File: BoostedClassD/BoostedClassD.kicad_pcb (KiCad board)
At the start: 4 copper layers, 82.2 x 58.4 mm, 83 parts, among them IC1 BQ25185, IC2 ESP32-WROOM-32UE-N8R2, IC5 INA236, J1 SYSTEM CONNECTOR 1, J2 SYSTEM CONNECTOR 2, J3 SPK OUT, J4 PROG, J5 CC, Q1 DMG3415U, U1 TPS631000, U2 TAS2320, U3 TAS2120, U4 TPS7A2018, U5 ATtiny412

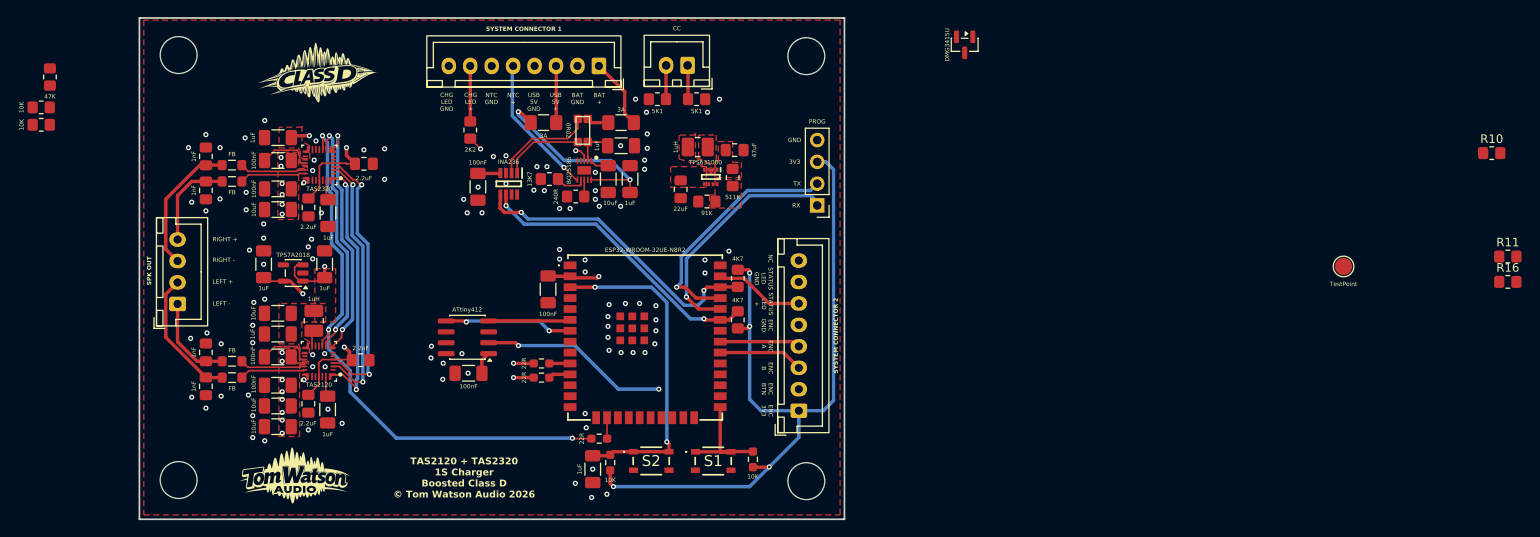
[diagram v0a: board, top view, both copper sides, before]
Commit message: more
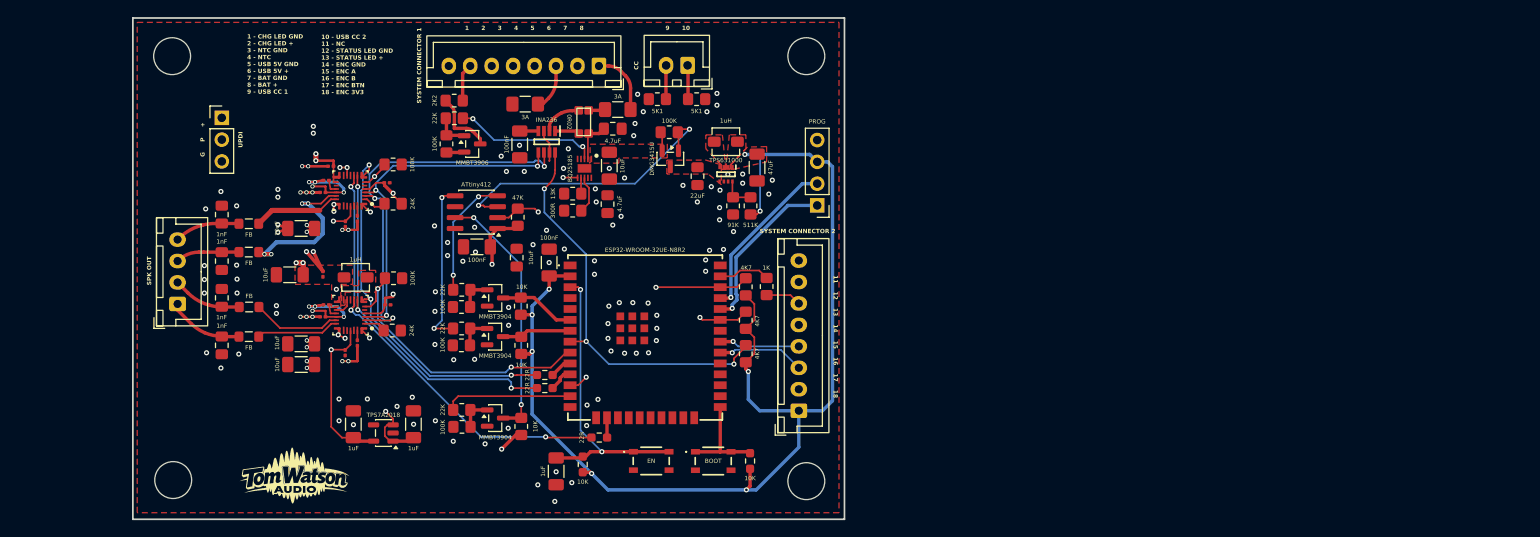
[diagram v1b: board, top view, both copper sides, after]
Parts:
- removed the G*** at (137.0, 78.2)
- removed R10: 0R*2, Resistor_SMD:R_0805_2012Metric_Pad1.20x1.40mm_HandSolder
- removed R11: 0R*3, Resistor_SMD:R_0805_2012Metric_Pad1.20x1.40mm_HandSolder
- removed TP1: TestPoint, TestPoint:TestPoint_Pad_D2.0mm
- added C32: 10uF, Capacitor_SMD:C_0805_2012Metric_Pad1.18x1.45mm_HandSolder, F.Cu at (160.3, 99.3)
- added J6: UPDI, Connector_PinHeader_2.54mm:PinHeader_1x03_P2.54mm_Vertical, F.Cu at (125.9, 83.0)
- added Q2: MMBT3904, Package_TO_SOT_SMD:SOT-23, F.Cu at (157.8, 104.0)
- added Q3: MMBT3904, Package_TO_SOT_SMD:SOT-23, F.Cu at (157.8, 108.5)
- added Q4: MMBT3904, Package_TO_SOT_SMD:SOT-23, F.Cu at (157.8, 118.0)
- added Q5: MMBT3906, Package_TO_SOT_SMD:SOT-23, F.Cu at (155.1, 86.0)
- added R22: 100K, Resistor_SMD:R_0805_2012Metric_Pad1.20x1.40mm_HandSolder, F.Cu at (145.9, 101.7)
- added R23: 100K, Resistor_SMD:R_0805_2012Metric_Pad1.20x1.40mm_HandSolder, F.Cu at (145.9, 88.4)
- added R24: 24K, Resistor_SMD:R_0805_2012Metric_Pad1.20x1.40mm_HandSolder, F.Cu at (145.8, 107.8)
- added R25: 24K, Resistor_SMD:R_0805_2012Metric_Pad1.20x1.40mm_HandSolder, F.Cu at (145.9, 93.0)
- added R26: 22K, Resistor_SMD:R_0805_2012Metric_Pad1.20x1.40mm_HandSolder, F.Cu at (153.9, 103.0)
- added R27: 100K, Resistor_SMD:R_0805_2012Metric_Pad1.20x1.40mm_HandSolder, F.Cu at (153.9, 105.1)
- added R28: 22K, Resistor_SMD:R_0805_2012Metric_Pad1.20x1.40mm_HandSolder, F.Cu at (153.9, 107.6)
- added R29: 100K, Resistor_SMD:R_0805_2012Metric_Pad1.20x1.40mm_HandSolder, F.Cu at (153.9, 109.5)
- added R30: 22K, Resistor_SMD:R_0805_2012Metric_Pad1.20x1.40mm_HandSolder, F.Cu at (153.9, 117.0)
- added R31: 100K, Resistor_SMD:R_0805_2012Metric_Pad1.20x1.40mm_HandSolder, F.Cu at (153.9, 119.0)
- added R32: 10K, Resistor_SMD:R_0805_2012Metric_Pad1.20x1.40mm_HandSolder, F.Cu at (160.8, 119.0)
- added R33: 4K7, Resistor_SMD:R_0805_2012Metric_Pad1.20x1.40mm_HandSolder, F.Cu at (187.0, 110.5)
- added R34: 1K, Resistor_SMD:R_0805_2012Metric_Pad1.20x1.40mm_HandSolder, F.Cu at (189.4, 102.7)
- added R35: 22K, Resistor_SMD:R_0805_2012Metric_Pad1.20x1.40mm_HandSolder, F.Cu at (153.0, 83.1)
- added R36: 100K, Resistor_SMD:R_0805_2012Metric_Pad1.20x1.40mm_HandSolder, F.Cu at (152.1, 86.0)
- C13, C14, C15, C16, C17, C18, C19, C20: footprint Capacitor_SMD:C_1206_3216Metric_Pad1.33x1.80mm_HandSolder -> Capacitor_SMD:C_0201_0603Metric
- C2: footprint Capacitor_SMD:C_0805_2012Metric_Pad1.18x1.45mm_HandSolder -> Capacitor_SMD:C_1206_3216Metric_Pad1.33x1.80mm_HandSolder
- C21, C22, C23, C24: footprint Capacitor_SMD:C_0805_2012Metric_Pad1.18x1.45mm_HandSolder -> Capacitor_SMD:C_0201_0603Metric
- C26, C27: value 1uF -> 4.7uF; footprint Capacitor_SMD:C_1206_3216Metric_Pad1.33x1.80mm_HandSolder -> Capacitor_SMD:C_0805_2012Metric_Pad1.18x1.45mm_HandSolder
- L1, L2: footprint Inductor_SMD:L_1008_2520Metric_Pad1.43x2.20mm_HandSolder -> Inductor_SMD:L_Vishay_IHLP-1212
- R17: value 240R -> 300R
- R18: value 13K7 -> 13K
- moved R16 99.3 mm to (178.1, 84.7), turned to 180 degrees
- moved R15 61.6 mm to (160.8, 109.5), turned to 90 degrees
- moved R14 60.5 mm to (160.8, 105.0), turned to 90 degrees
- moved R13 56.9 mm to (160.4, 94.6), turned to 90 degrees
- moved Q1 36.8 mm to (178.2, 87.8)
- moved U4 21.4 mm to (144.8, 119.7)
- moved C5 21.4 mm to (141.3, 118.7)
- moved C6 21.3 mm to (148.3, 118.7)
- moved C8 14.8 mm to (155.7, 98.0)
- moved U5 14.6 mm to (155.6, 94.0)
- moved C29 12.3 mm to (125.9, 99.7), turned to 90 degrees
- moved FB2 10.3 mm to (129.1, 98.7)
- moved C14 9.54 mm to (137.7, 106.2)
- moved C20 8.74 mm to (137.7, 101.2), turned to 90 degrees
- moved C16 8.50 mm to (141.7, 109.2)
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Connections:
- C2 pad 1: /ENC 3V3 -> /ESP3V3
- C22 pad 1: /Amplifiers/VDD1V8 -> /ESP3V3
- C24 pad 1: /Amplifiers/VDD1V8 -> /ESP3V3
- C25 pad 1: /CHGPOWER/BQ-SYS -> /BQ-SYS
- C3 pad 1: /ENC 3V3 -> /ESP3V3
- C7 pad 1: /ENC 3V3 -> /ESP3V3
- C8 pad 1: /Amplifiers/SYS -> /BQ-SYS
- IC1 pad 1: /CHGPOWER/BQ-SYS -> /BQ-SYS
- IC1 pad 3: Net-(IC1-STAT2) -> /CHGPOWER/STAT2_N
- IC2 pad 12: /Amplifiers/SDOUT -> /Amplifiers/AMP2320_SDZ
- IC2 pad 13: unconnected-(IC2-IO14-Pad13) -> /ESP32-ATTINY/SHUTDOWN_ACK
- IC2 pad 2: /ENC 3V3 -> /ESP3V3
- IC2 pad 37: /STATUS LED + -> Net-(IC2-IO23)
- IC2 pad 8: /ESP32-ATTINY/ALERT -> /ALERT_N
- IC2 pad 9: unconnected-(IC2-IO33-Pad9) -> /AMP2120_SDZ
- IC5 pad 4: /ENC 3V3 -> /ESP3V3
- IC5 pad 7: Net-(IC5-A0) -> GND
- IC5 pad 8: /CHGPOWER/ALERT -> /ALERT_N
- J2 pad 1: /ENC 3V3 -> /ESP3V3
- J3 pad 1: /LEFT - -> /LEFT +
- J3 pad 2: /LEFT + -> /LEFT -
- J4 pad 3: /ENC 3V3 -> /ESP3V3
- Q1 pad 2: /CHGPOWER/BQ-SYS -> /BQ-SYS
- R1 pad 1: /ENC 3V3 -> /ESP3V3
- R12 pad 1: /ENC 3V3 -> /ESP3V3
- R13 pad 1: /Amplifiers/SYS -> /BQ-SYS
- R14 pad 1: /ENC 3V3 -> /ESP3V3
- R15 pad 1: /ENC 3V3 -> /ESP3V3
- R16 pad 2: /CHGPOWER/BQ-SYS -> /BQ-SYS
- R19 pad 1: Net-(IC1-STAT2) -> Net-(Q5-C)
- R2 pad 1: /ENC 3V3 -> /ESP3V3
- R7 pad 1: /ENC 3V3 -> /ESP3V3
- R8 pad 1: /ENC 3V3 -> /ESP3V3
- U1 pad 1: /ENC 3V3 -> /ESP3V3
- U2 pad 16: unconnected-(U2-HW_SEL1-Pad16) -> GND
- U2 pad 2: unconnected-(U2-HW_SEL4_AD1-Pad2) -> /Amplifiers/ADDR2320
- U2 pad 22: unconnected-(U2-VSNSP-Pad22) -> GND
- U2 pad 23: unconnected-(U2-VSNSN-Pad23) -> GND
- U2 pad 5: /Amplifiers/VDD1V8 -> /ESP3V3
- U2 pad 7: unconnected-(U2-SD_N-Pad7) -> /Amplifiers/AMP2320_SDZ
- U3 pad 16: unconnected-(U3-HW_SEL1-Pad16) -> GND
- U3 pad 2: unconnected-(U3-HW_SEL4_AD1-Pad2) -> /Amplifiers/ADDR2120
- U3 pad 22: unconnected-(U3-VSNSP-Pad22) -> GND
- U3 pad 23: unconnected-(U3-VSNSN-Pad23) -> GND
- U3 pad 5: /Amplifiers/VDD1V8 -> /ESP3V3
- U3 pad 7: unconnected-(U3-SD_N-Pad7) -> /AMP2120_SDZ
- U5 pad 1: /Amplifiers/SYS -> /BQ-SYS
- U5 pad 4: /ESP32-ATTINY/PLAY_PAUSE -> /ESP32-ATTINY/PLAY_DRIVE
- U5 pad 5: /ESP32-ATTINY/POWER_OFF_REQ -> /ESP32-ATTINY/OFF_REQ_DRIVE
- U5 pad 7: Net-(U5-PA3) -> /ESP32-ATTINY/ACK_N
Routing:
- net /ESP3V3: track 0.00 -> 183.9 mm, vias 0 -> 10
- net /ENC 3V3: track 115.8 -> 0.00 mm, vias 5 -> 0
- net /ALERT_N: track 0.00 -> 47.4 mm, vias 0 -> 3
- net GND: track 0.00 -> 44.7 mm, vias 107 -> 125
- net /Amplifiers/SCL: track 114.8 -> 72.1 mm
- net /Amplifiers/AMP2320_SDZ: track 0.00 -> 41.5 mm, vias 0 -> 2
- net /BQ-SYS: track 0.00 -> 40.4 mm, vias 0 -> 2
- net /CHGPOWER/POWER-ON-MOSFET: track 0.00 -> 34.4 mm, vias 0 -> 2
- net /AMP2120_SDZ: track 0.00 -> 34.2 mm, vias 0 -> 2
- net /Amplifiers/SDA: track 110.1 -> 78.5 mm
- net /ESP32-ATTINY/ACK_N: track 0.00 -> 29.9 mm, vias 0 -> 2
- net /Amplifiers/PVDD: track 1.87 -> 29.6 mm
- net /USB5V +: track 24.5 -> 0.00 mm, vias 2 -> 0
- net /Amplifiers/SYS: track 28.7 -> 50.6 mm, vias 2 -> 6
- net /Amplifiers/VDD1V8: track 57.2 -> 37.2 mm, vias 3 -> 2
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- added copper zone on F.Cu, net /BQ-SYS
- added copper zone on F.Cu, net /ESP3V3
- added copper zone on F.Cu, net Net-(U3-SW)
- removed copper zone on F.Cu, net /Amplifiers/PVDD
- removed copper zone on F.Cu, net /ENC 3V3
- removed copper zone on F.Cu, net Net-(U1-FB)
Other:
- board size 82.2 x 58.4 mm -> 82.9 x 58.4 mm
- board text added: "1 - CHG LED GND 2 - CHG LED + 3 - NTC GND 4 - NTC 5 - USB 5V GND 6 - USB 5V + 7 - BAT GND 8 - BAT + 9 - USB CC 1"
- board text added: "1 2 3 4 5 6 7 8"
- board text added: "10 - USB CC 2 11 - NC 12 - STATUS LED GND 13 - STATUS LED + 14 - ENC GND 15 - ENC A 16 - ENC B 17 - ENC BTN 18 - ENC 3V3"
- board text added: "11 12 13 14 15 16 17 18"
- board text added: "9 10"
- board text added: "G P +"
